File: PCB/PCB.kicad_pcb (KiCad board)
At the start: 6 copper layers, 255 x 147 mm, 168 parts, among them IC1 S25FL256LAGMFI003, IC2 LT1932ES6#TRMPBF, J1 0878311420, J2 USB_B_Micro, J3 FTS-102-02-F-DV-TR, J4 62684-402100ALF, J5 L77HDE15SD1CH4FVGA, J6 USB1130-15-A_REVA, J7 FTSH-104-01-F-DV, SW1 SW_Push, SW2 SW_Push, SW3 SW_Push, SW4 SW_Push, U1 TPS54325, U2 TPS54294, U3 COM-09032, U4 XC7A100T-FTG256, U5 IS62C1024AL-35QLI-TR, Y1 Crystal_GND24, Y2 ECS-3953M-400-BN-TR

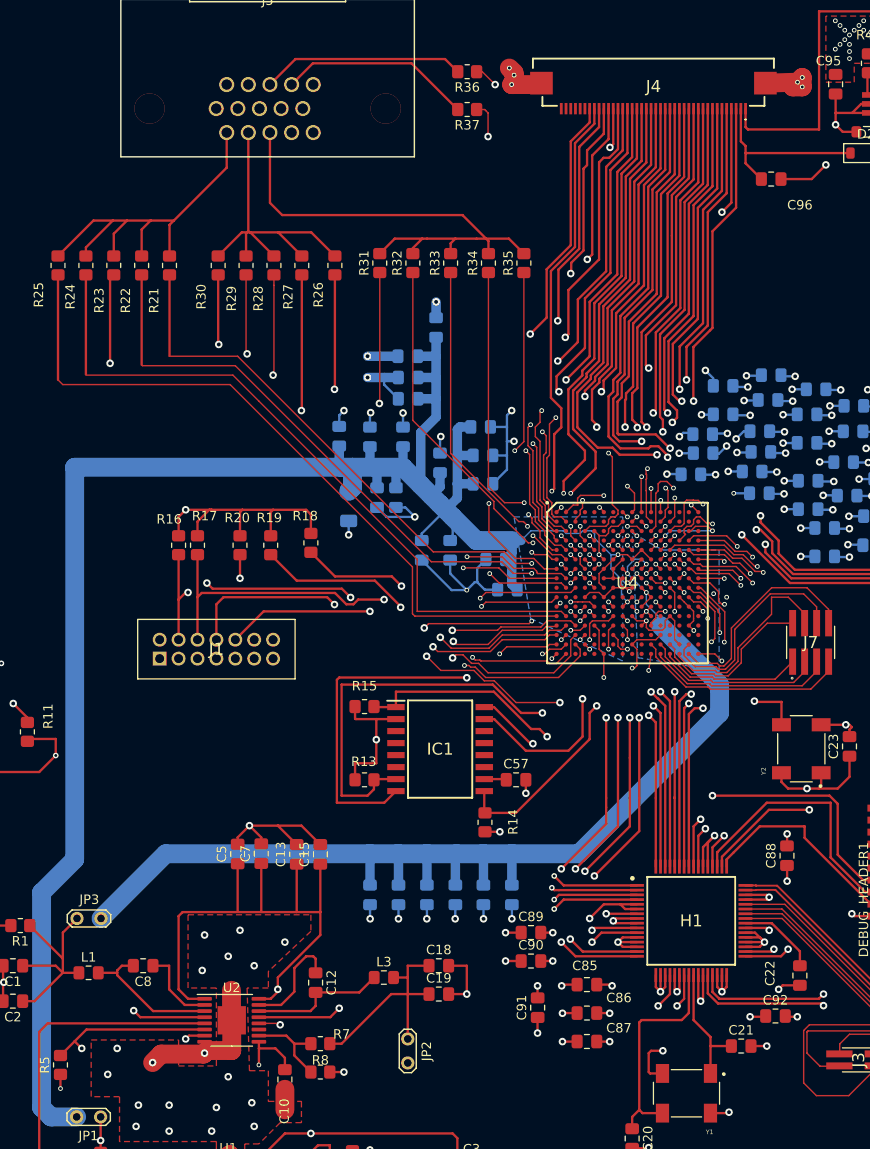
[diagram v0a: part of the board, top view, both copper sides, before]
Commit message: start fix routing
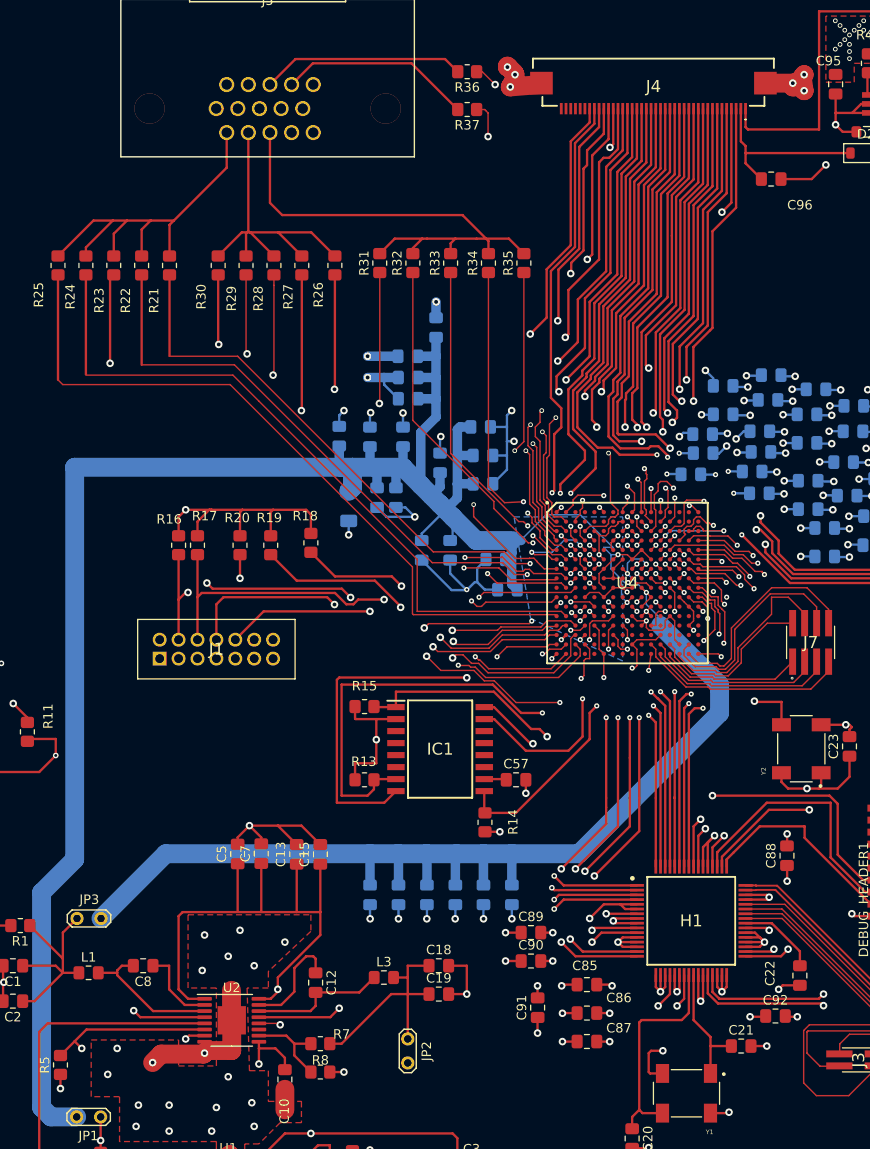
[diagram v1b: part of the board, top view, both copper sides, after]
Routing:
- net GND: track 478.3 -> 484.8 mm, vias 210 -> 209
- net +3.3V: track 242.8 -> 248.4 mm
- net /FPGA/GPIO0: track 67.2 -> 70.9 mm
- net /FPGA/GPIO1: track 73.7 -> 77.3 mm
- net /FPGA/MOSI: track 61.3 -> 64.6 mm
- net Net-(U4A-IO_L15P_T2_DQS_15): track 79.5 -> 82.6 mm
- net Net-(U4C-TDO_0): track 52.9 -> 56.0 mm
- net +1V0: track 223.0 -> 226.0 mm
- net /FPGA/BLUE4: track 48.3 -> 51.2 mm
- net /FPGA/GPIO4: track 86.6 -> 89.5 mm
- net /FPGA/GPIO6: track 86.2 -> 89.0 mm
- net /FPGA/GPIO2: track 79.5 -> 82.2 mm
- net /FPGA/GPIO3: track 85.3 -> 87.9 mm
- net /FPGA/GPIO5: track 93.4 -> 96.0 mm
- net Net-(IC1-SCK): track 68.3 -> 66.4 mm
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- removed copper zone on B.Cu, net +1V8

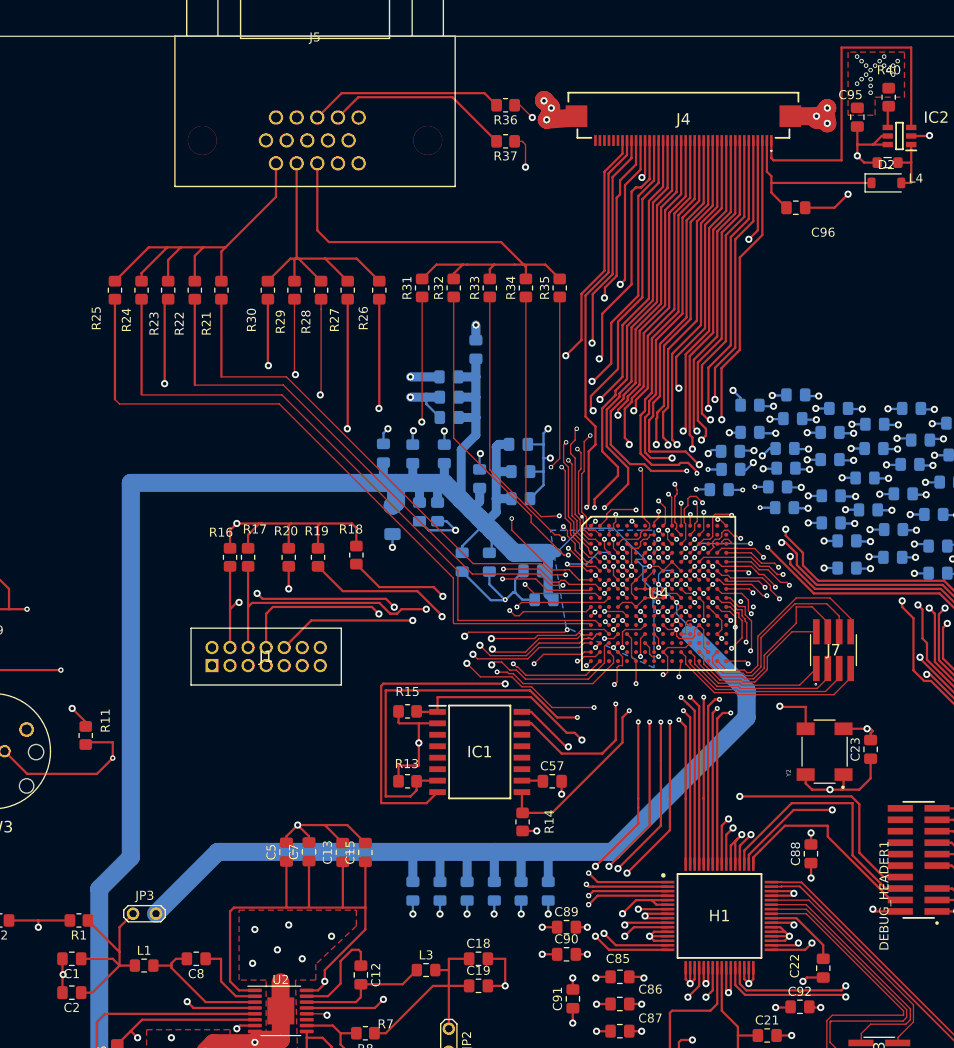
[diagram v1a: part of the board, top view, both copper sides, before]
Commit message: Correct mistakes
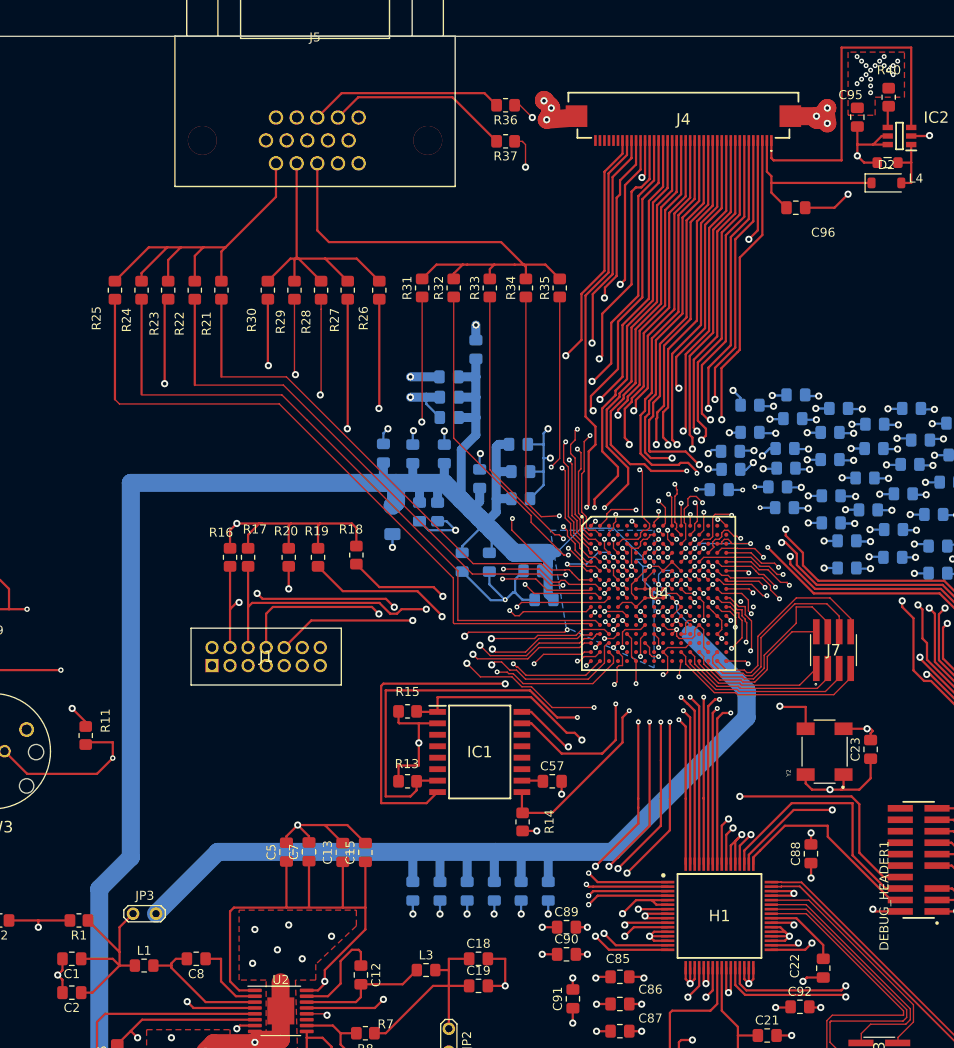
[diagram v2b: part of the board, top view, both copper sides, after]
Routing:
- net Net-(U2-VFB1): track 38.4 -> 39.5 mm
- net Net-(U4A-IO_L13P_T2_MRCC_15): track 63.4 -> 64.0 mm
- net Net-(U4A-IO_L16P_T2_A28_15): track 60.8 -> 61.4 mm
- net GND: track 484.8 -> 485.3 mm
